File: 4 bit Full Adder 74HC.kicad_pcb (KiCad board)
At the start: 2 copper layers, 69 x 67.5 mm, 31 parts, among them J1 Screw_Terminal_01x02, J2 Screw_Terminal_01x02, SW1 SW_DIP_x04, SW2 SW_DIP_x04, SW3 SW_DIP_x01, U1 74HC86, U2 74HC86, U3 74LS08, U5 74LS32, U6 74LS08

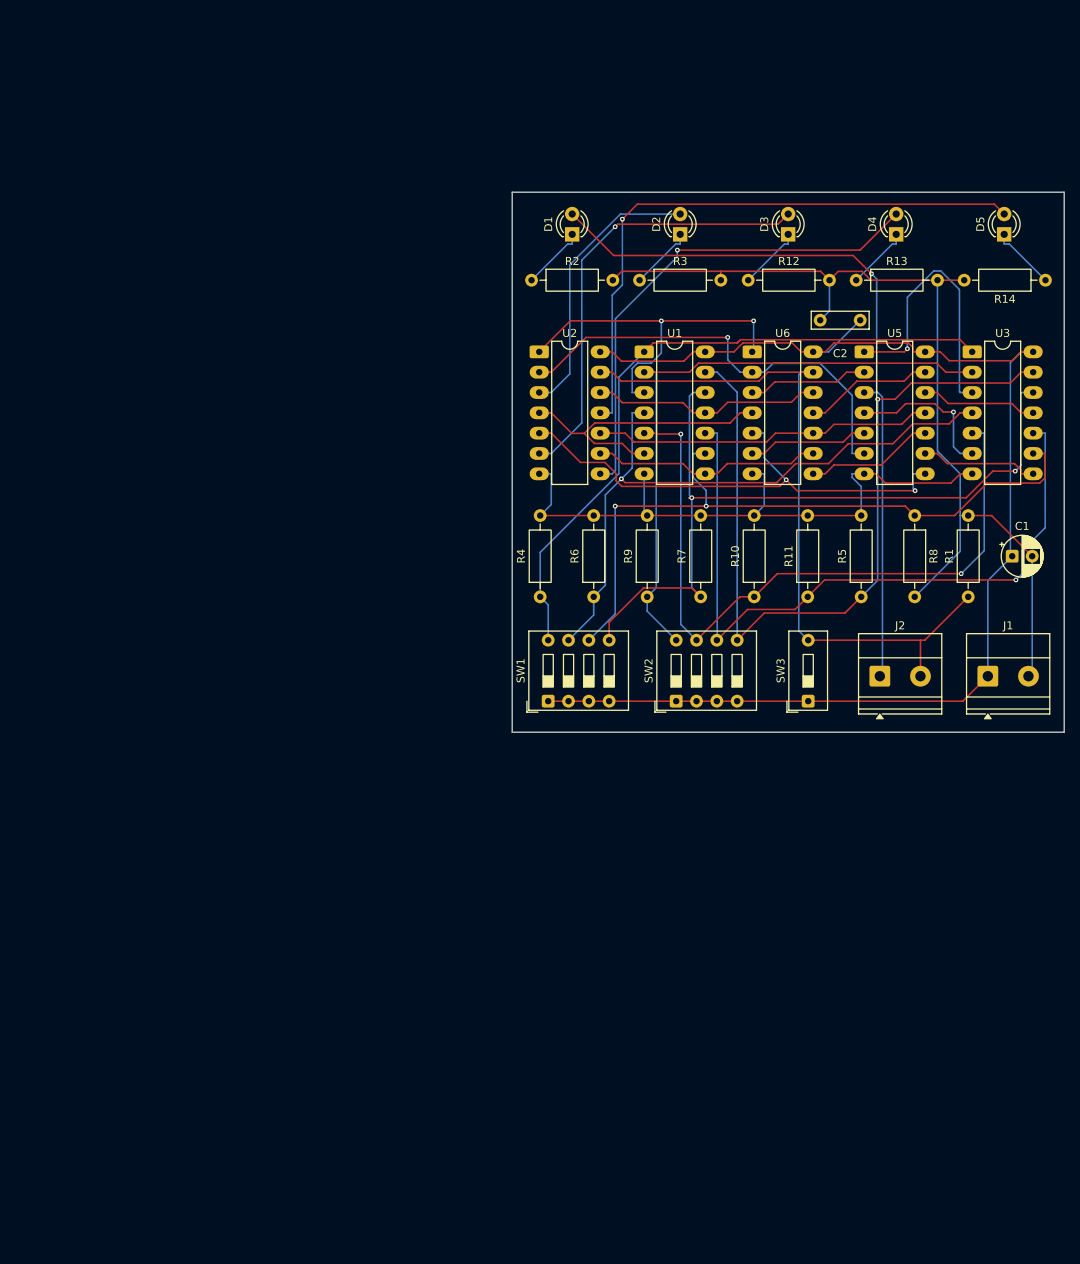
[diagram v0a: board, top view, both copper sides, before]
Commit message: Update PCB
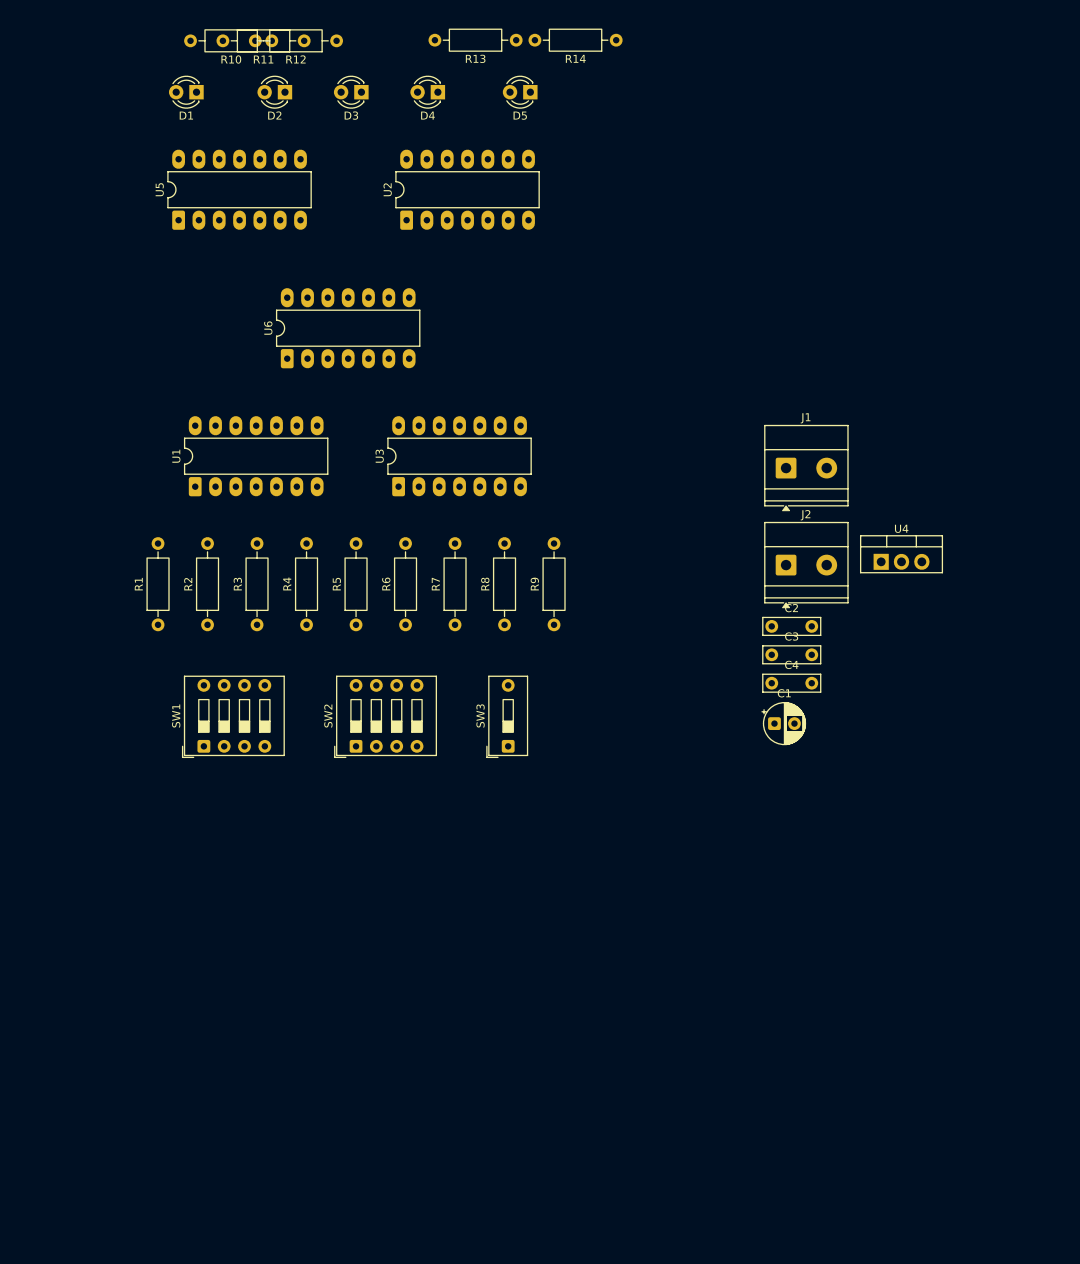
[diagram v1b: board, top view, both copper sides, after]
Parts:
- added C3: 0.1uF, Capacitor_THT:C_Rect_L7.0mm_W2.0mm_P5.00mm, F.Cu at (134.9, 101.3)
- added C4: 0.33uF, Capacitor_THT:C_Rect_L7.0mm_W2.0mm_P5.00mm, F.Cu at (134.9, 104.9)
- added U4: LM7805_TO220, Package_TO_SOT_THT:TO-220-3_Vertical, F.Cu at (148.6, 89.7)
- R10, R11: value 10k -> 220
- R2, R3: value 220 -> 10k
- moved R1 101.3 mm to (58.2, 97.6)
- moved R11 93.8 mm to (76.5, 24.6), turned to 180 degrees
- moved R10 92.0 mm to (72.5, 24.6), turned to 180 degrees
- moved U5 87.3 mm to (60.8, 47.0), turned to 90 degrees
- moved U3 73.7 mm to (88.3, 80.3), turned to 90 degrees
- moved R3 64.4 mm to (70.6, 97.6), turned to 90 degrees
- moved R5 63.2 mm to (83.0, 97.6)
- moved D5 61.8 mm to (104.8, 31.0), turned to 180 degrees
- moved R14 61.5 mm to (115.5, 24.5)
- moved D4 60.0 mm to (93.2, 31.0), turned to 180 degrees
- moved R12 59.5 mm to (80.5, 24.6), turned to 180 degrees
- moved R2 59.1 mm to (64.4, 97.6), turned to 90 degrees
- moved U1 58.6 mm to (62.9, 80.3), turned to 90 degrees
- moved U6 58.1 mm to (74.4, 64.3), turned to 90 degrees
- moved D3 56.2 mm to (83.7, 31.0), turned to 180 degrees
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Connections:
- net Net-(J2-Pin_2) renamed Ci
- D5 pad 2: Net-(D5-A) -> Co
- J1 pad 1: +5V -> Net-(J1-Pin_1)
- J2 pad 1: Net-(D1-A) -> Co
- R10 pad 1: Net-(R10-Pad1) -> Net-(D1-K)
- R11 pad 1: Net-(R11-Pad1) -> Net-(D2-K)
- R2 pad 1: Net-(D1-K) -> Net-(R2-Pad1)
- R3 pad 1: Net-(D2-K) -> Net-(R3-Pad1)
- SW1 pad 5: Net-(R7-Pad1) -> Net-(R2-Pad1)
- SW1 pad 6: Net-(R8-Pad1) -> Net-(R4-Pad1)
- SW1 pad 8: Net-(R4-Pad1) -> Net-(R8-Pad1)
- SW2 pad 5: Net-(R5-Pad1) -> Net-(R3-Pad1)
- SW2 pad 6: Net-(R11-Pad1) -> Net-(R5-Pad1)
- SW2 pad 7: Net-(R10-Pad1) -> Net-(R7-Pad1)
- U1 pad 1: Net-(R4-Pad1) -> Net-(R8-Pad1)
- U1 pad 10: Net-(R11-Pad1) -> Net-(R5-Pad1)
- U1 pad 12: Net-(R7-Pad1) -> Net-(R2-Pad1)
- U1 pad 13: Net-(R5-Pad1) -> Net-(R3-Pad1)
- U1 pad 5: Net-(R10-Pad1) -> Net-(R7-Pad1)
- U1 pad 9: Net-(R8-Pad1) -> Net-(R4-Pad1)
- U2 pad 11: Net-(D5-A) -> Net-(D1-A)
- U2 pad 3: Net-(D2-A) -> Net-(D4-A)
- U2 pad 8: Net-(D4-A) -> Net-(D2-A)
- U3 pad 1: Net-(R4-Pad1) -> Net-(R8-Pad1)
- U3 pad 10: Net-(R11-Pad1) -> Net-(R5-Pad1)
- U3 pad 12: Net-(R7-Pad1) -> Net-(R2-Pad1)
- U3 pad 13: Net-(R5-Pad1) -> Net-(R3-Pad1)
- U3 pad 5: Net-(R10-Pad1) -> Net-(R7-Pad1)
- U3 pad 9: Net-(R8-Pad1) -> Net-(R4-Pad1)
- U5 pad 3: Net-(D1-A) -> Co
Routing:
- net GND: track 204.9 -> 0.00 mm
- net +5V: track 165.9 -> 0.00 mm
- net Net-(R5-Pad1): track 100.2 -> 0.00 mm, vias 1 -> 0
- net Net-(R7-Pad1): track 98.7 -> 0.00 mm, vias 2 -> 0
- net Net-(D1-A): track 93.2 -> 0.00 mm, vias 1 -> 0
- net Ci: track 89.9 -> 0.00 mm
- net Net-(R11-Pad1): track 89.3 -> 0.00 mm, vias 1 -> 0
- net Net-(R10-Pad1): track 88.0 -> 0.00 mm, vias 2 -> 0
- net Net-(R8-Pad1): track 87.8 -> 0.00 mm, vias 2 -> 0
- net Net-(R4-Pad1): track 84.3 -> 0.00 mm
- net Net-(R6-Pad1): track 80.9 -> 0.00 mm, vias 1 -> 0
- net Net-(R9-Pad1): track 78.9 -> 0.00 mm
- net Net-(D5-A): track 75.2 -> 0.00 mm, vias 1 -> 0
- net Net-(U2-Pad5): track 63.3 -> 0.00 mm, vias 2 -> 0
- net Net-(D4-A): track 62.1 -> 0.00 mm, vias 1 -> 0
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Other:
- board outline removed

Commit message: Update PCB
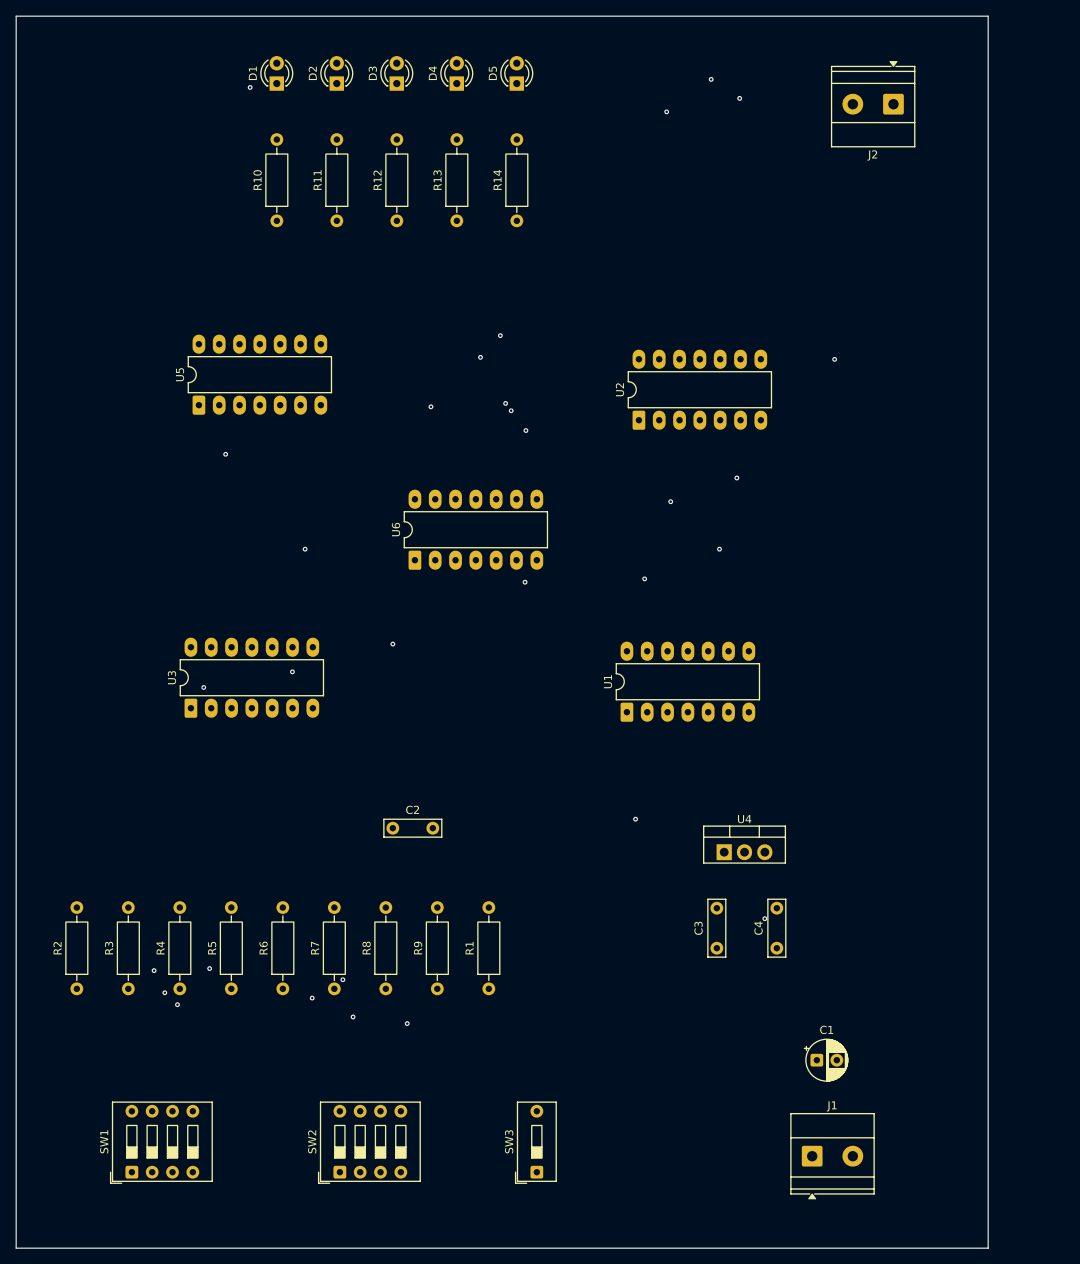
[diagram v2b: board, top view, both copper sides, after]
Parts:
- moved J1 86.1 mm to (140.0, 164.0)
- moved R1 61.5 mm to (99.6, 143.1)
- moved U1 60.9 mm to (116.8, 108.5)
- moved J2 59.2 mm to (150.2, 32.5), turned to 180 degrees
- moved SW1 54.0 mm to (55.0, 166.0)
- moved C2 53.7 mm to (87.6, 123.0)
- moved SW3 53.4 mm to (105.6, 166.0)
- moved SW2 53.3 mm to (81.0, 166.0)
- moved R2 48.3 mm to (48.1, 143.1)
- moved R3 48.3 mm to (54.5, 143.1)
- moved R4 48.2 mm to (61.0, 143.1)
- moved R5 48.1 mm to (67.4, 143.1)
- moved R6 48.0 mm to (73.8, 143.1)
- moved R7 47.9 mm to (80.3, 143.1)
- moved R8 47.9 mm to (86.7, 143.1)
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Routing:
- net Net-(U5-Pad5): vias 0 -> 2
- net Net-(U5-Pad13): vias 0 -> 1
- net Net-(U5-Pad10): vias 0 -> 1
- net Net-(U2-Pad5): vias 0 -> 1
- net Net-(U2-Pad2): vias 0 -> 1
- net Net-(U2-Pad10): vias 0 -> 1
- net Net-(U1-Pad8): vias 0 -> 1
- net Net-(U1-Pad6): vias 0 -> 1
- net Net-(U1-Pad3): vias 0 -> 1
- net Net-(U1-Pad11): vias 0 -> 1
- net Net-(R9-Pad1): vias 0 -> 2
- net Net-(R8-Pad1): vias 0 -> 1
- net Net-(R6-Pad1): vias 0 -> 1
- net Net-(R5-Pad1): vias 0 -> 1
- net Net-(R4-Pad1): vias 0 -> 2
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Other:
- board outline added: 121.5 x 154 mm
